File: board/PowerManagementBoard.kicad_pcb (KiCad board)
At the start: 2 copper layers, 168.9 x 115.6 mm, 162 parts, among them IC1 ACS37010LLZATR-030B3, IC2 ACS37010LLZATR-030B3, IC3 ACS37010LLZATR-030B3, IC4 ACS37010LLZATR-030B3, IC6 ACS37010LLZATR-030B3, J1 RJ45_LED_Shielded, J10 768250002, J11 768250002, J12 768250002, J13 768250002, J14 768250002, J15 768250002, J16 768250002, J17 768250002, J18 768250002, J2 SS-73100-082, J3 SS-73100-082, J5 768250002, J6 768250002, J7 768250002, J8 768250002, J9 768250002, Q1 BSS138, Q2 IPB180N10S4-02, Q3 Si4162DY, Q4 IPB180N10S4-02, Q5 Si4162DY, Q6 Si4162DY, Q7 Si4162DY, Q8 Si4162DY, Q9 IPB180N10S4-02, U1 LT1910, U10 ACS72981LLRATR-100U3, U11 LT1910, U12 LT1910, U13 LT1910, U14 LT1910, U15 Teensy4.1_DEV-16771, U16 OKI-78SR-3.3_1.5-W36H-C, U17 OKI-78SR-5_1.5-W36H-C, U19 LT1910, U2 LM5050MK-1_NOPB, U3 LM5050MK-1_NOPB, U4 Opamp_Dual, U5 Opamp_Dual, U6 Opamp_Dual

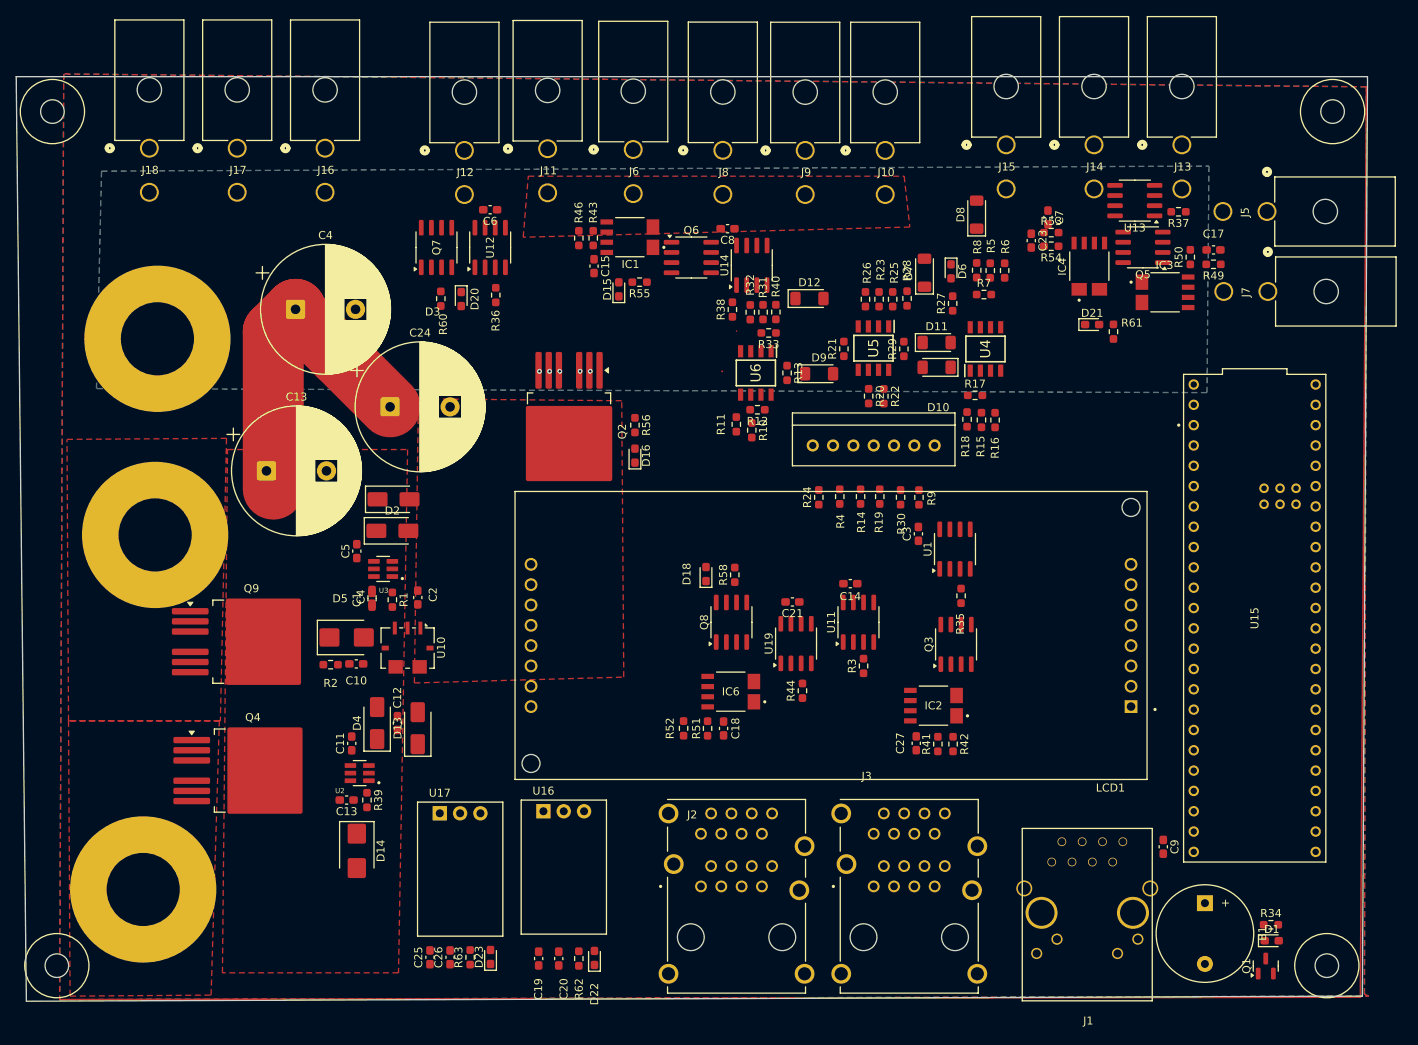
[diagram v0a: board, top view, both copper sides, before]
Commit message: Most Traces done
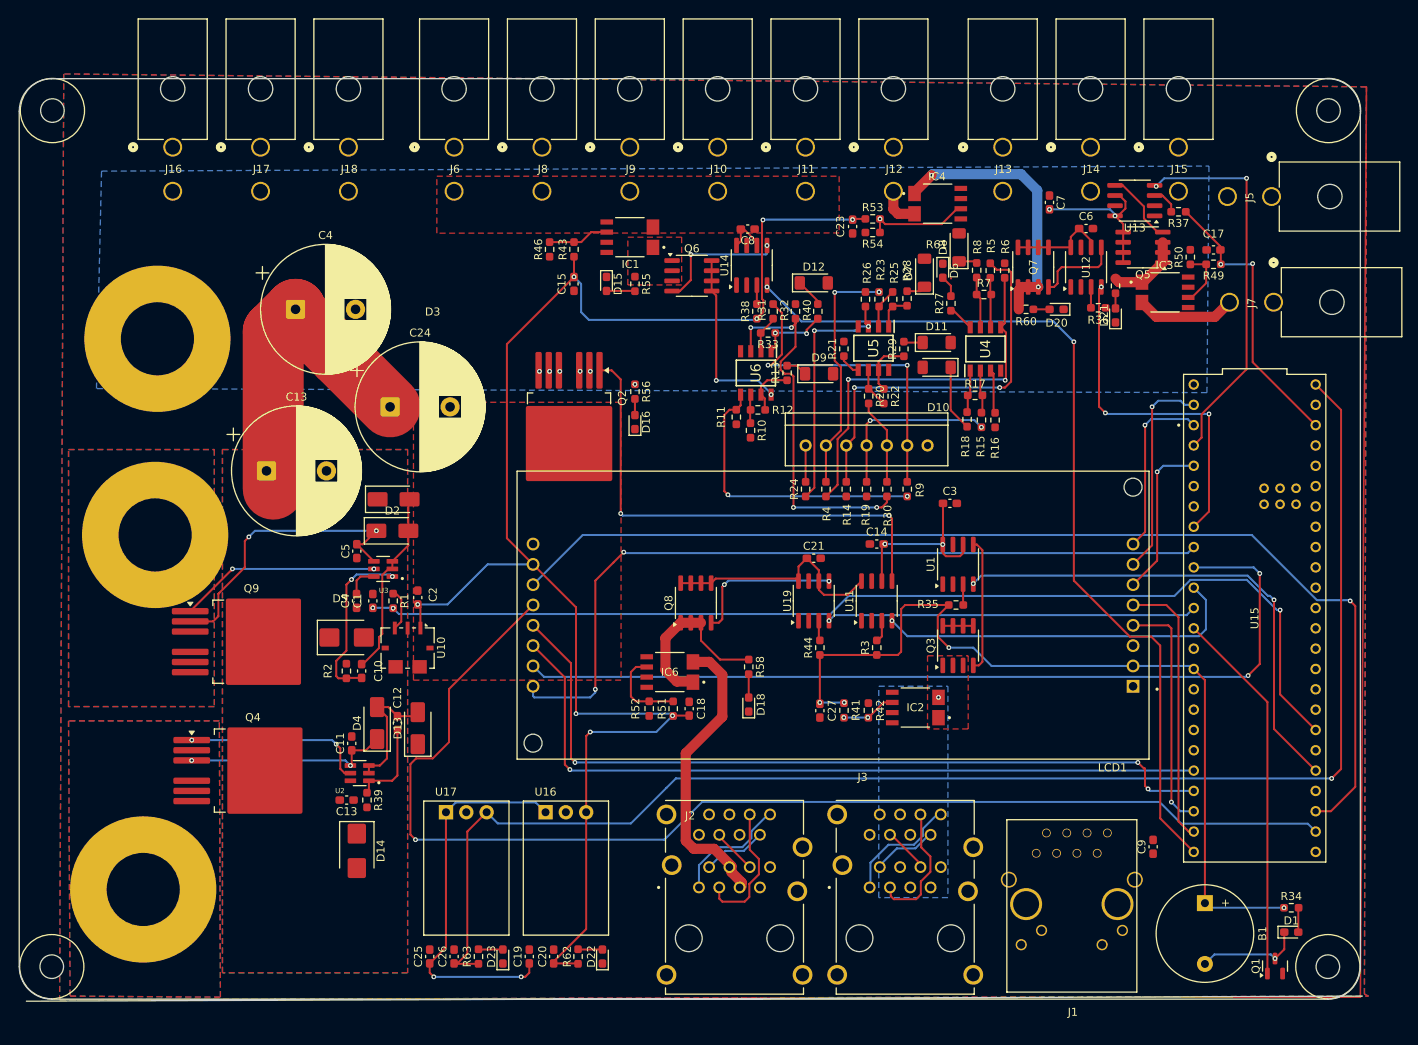
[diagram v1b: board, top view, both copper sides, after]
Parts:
- moved R36 75.3 mm to (168.9, 60.6), turned to 180 degrees
- moved Q7 74.6 mm to (160.8, 55.6)
- moved U12 74.5 mm to (167.4, 55.6)
- moved C6 74.5 mm to (167.4, 50.7)
- moved D20 74.4 mm to (163.7, 60.8), turned to 180 degrees
- moved R60 73.2 mm to (159.9, 60.8), turned to 0 degrees
- moved J12 53.6 mm to (143.3, 40.6)
- moved J11 32.2 mm to (132.3, 40.6)
- moved J18 24.9 mm to (75.2, 40.6)
- moved J8 22.6 mm to (99.4, 40.6)
- moved C23 22.4 mm to (138.2, 50.5)
- moved J6 22.4 mm to (88.4, 40.6)
- moved J13 22.4 mm to (157.0, 40.6)
- moved R53 22.4 mm to (140.7, 49.5)
- moved R54 22.4 mm to (140.7, 51.2)
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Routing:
- net +3V3: track 0.00 -> 340.9 mm, vias 0 -> 14
- net +5V: track 0.07 -> 183.5 mm, vias 0 -> 1
- net +24V: track 0.00 -> 167.1 mm, vias 0 -> 8
- net /LCD/D6: track 0.00 -> 153.2 mm, vias 0 -> 1
- net /LCD/D7: track 0.00 -> 137.8 mm, vias 0 -> 1
- net /Current Protection/BattVout: track 0.00 -> 133.9 mm, vias 0 -> 3
- net /Switching Circuit/LC_EN: track 0.00 -> 112.7 mm, vias 0 -> 2
- net /LCD/D3: track 0.00 -> 111.9 mm, vias 0 -> 2
- net /LCD/D2: track 0.00 -> 100.0 mm, vias 0 -> 2
- net /LCD/D5: track 0.00 -> 99.4 mm, vias 0 -> 3
- net /LCD/D4: track 0.00 -> 95.4 mm, vias 0 -> 1
- net /Switching Circuit/M2_EN: track 0.00 -> 62.8 mm, vias 0 -> 2
- net Net-(Q2-G): track 0.00 -> 61.9 mm, vias 0 -> 2
- net Net-(Conn1-Pad3): track 0.00 -> 48.8 mm, vias 0 -> 2
- net Net-(U4B-+): track 0.00 -> 48.8 mm, vias 0 -> 2
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- added copper zone on F.Cu, net /Current-Sensinator/LCin
- added copper zone on F.Cu, net /Current-Sensinator/m2in
- added copper zone on B.Cu, net /Current-Sensinator/m2out
- added copper zone on B.Cu, net Net-(D14-K)
- added copper zone on B.Cu, net Net-(D2-K)
- added copper zone on B.Cu, net Net-(D4-K)
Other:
- board size 168.9 x 115.6 mm -> 167.9 x 115.3 mm
